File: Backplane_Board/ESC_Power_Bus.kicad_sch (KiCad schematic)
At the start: 19 parts, among them Q2 ZXMN3A14F, SW2 SW_DPST_x2

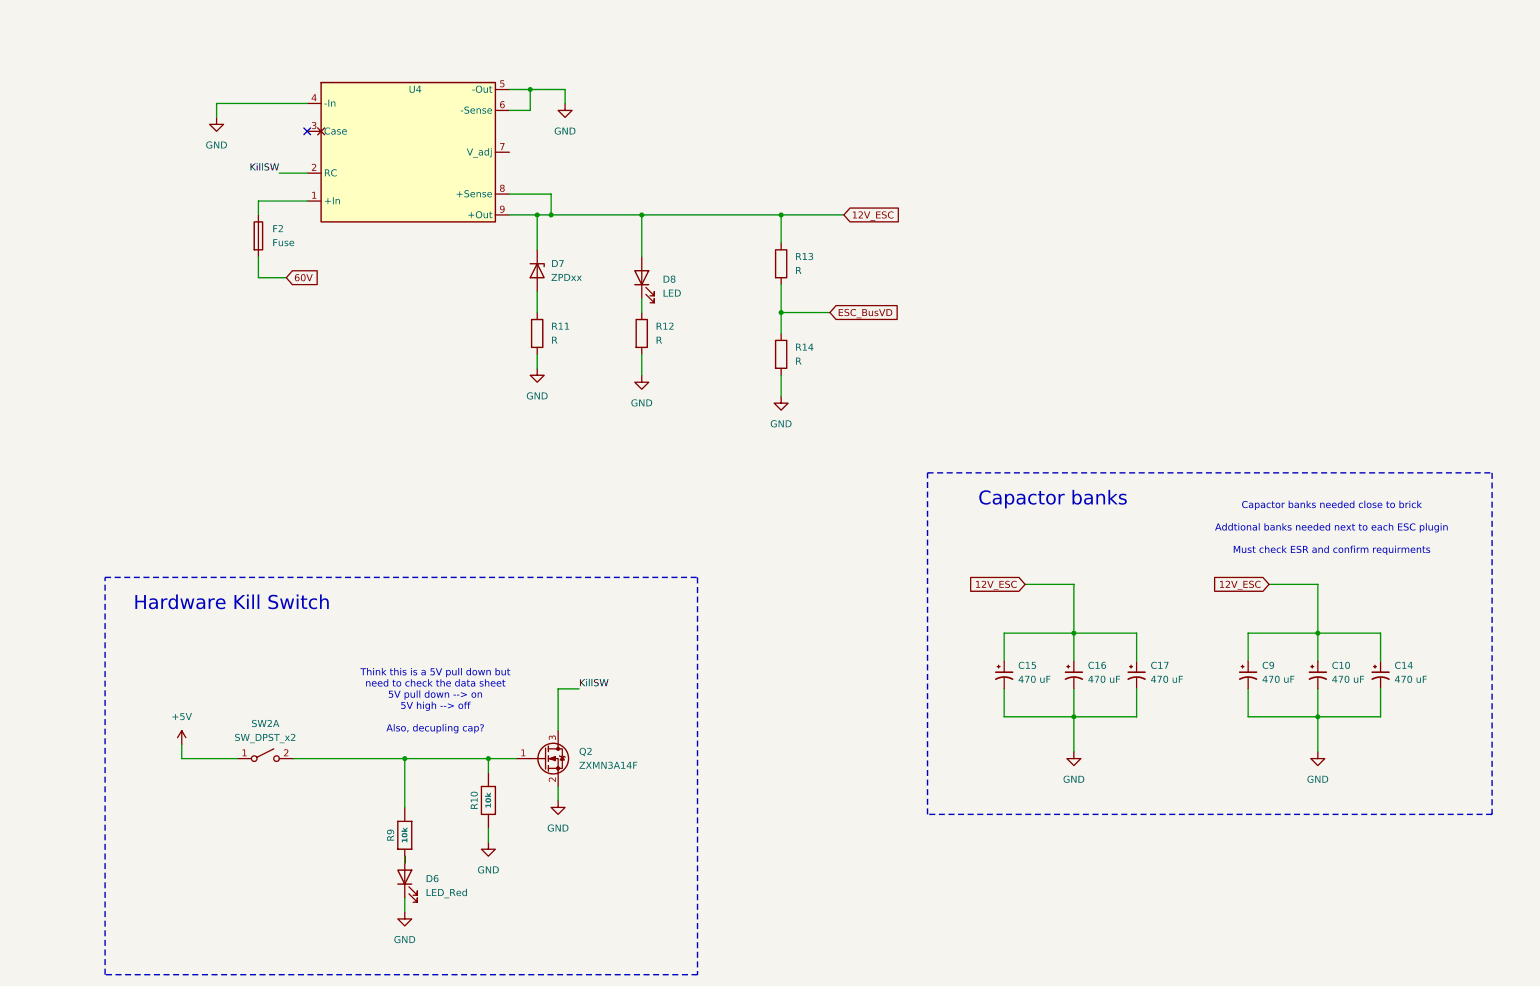
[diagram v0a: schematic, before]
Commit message: backup before heavy revtion
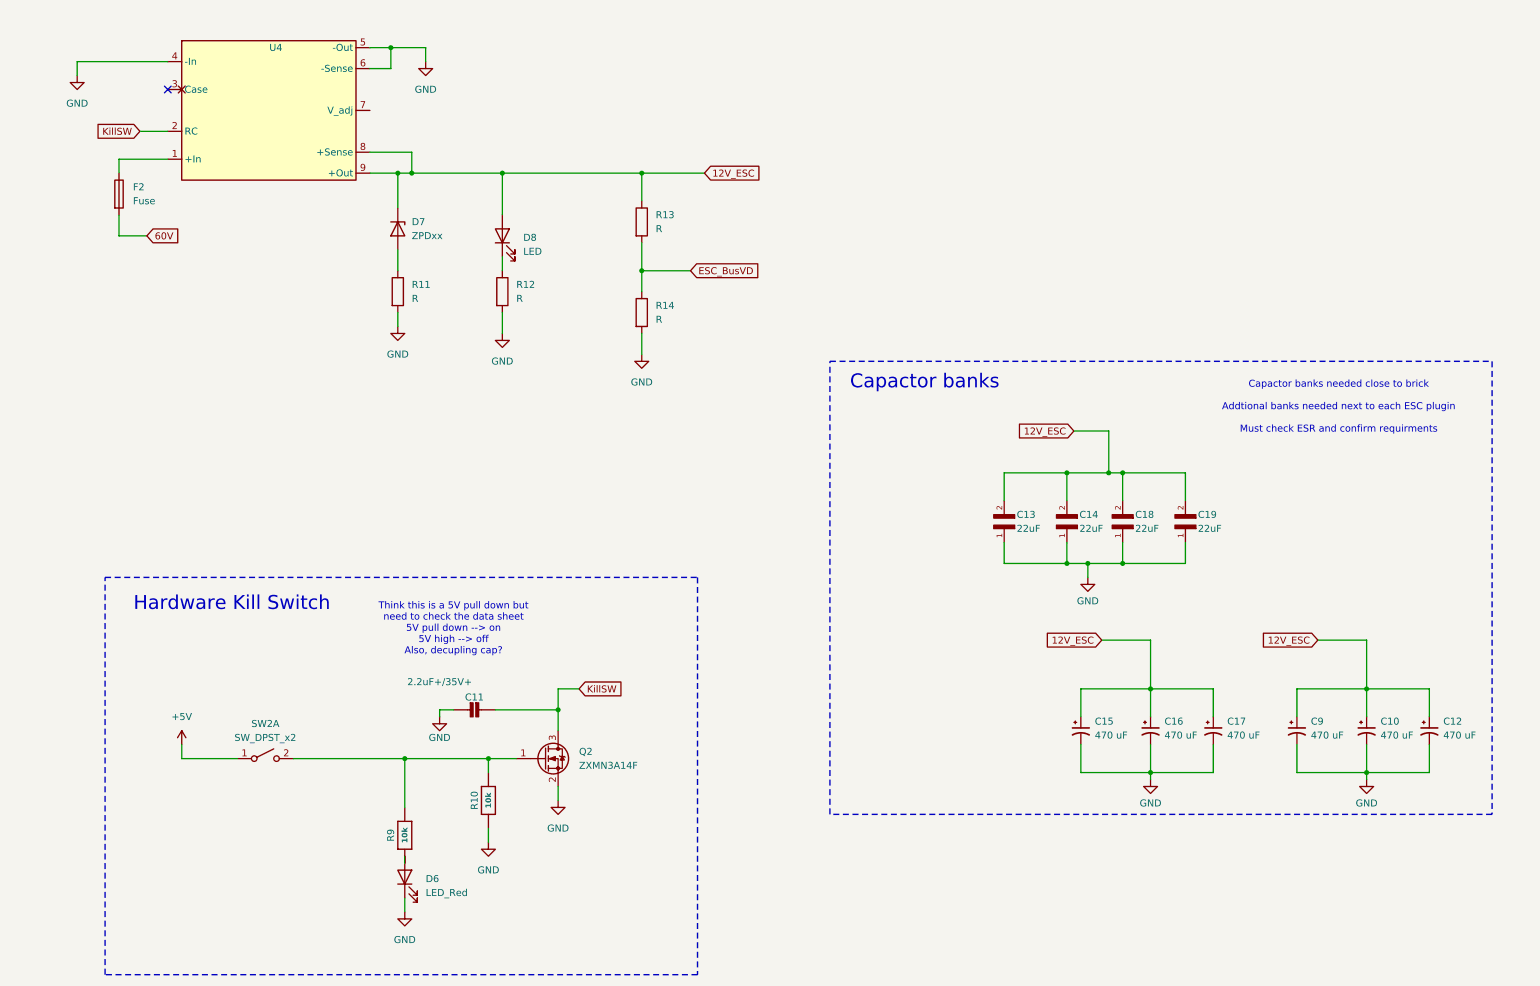
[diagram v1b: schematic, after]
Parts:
- removed C14: 470 uF, 470UF CAP:CAP_EEHZU1V471V, symbol Device:C_Polarized_Small_US
- added C11: 2.2uF+/35V+, Capacitor_SMD:C_0805_2012Metric, symbol Adafruit MOSFET Driver STEMMA Breakout-eagle-import:CAP_CERAMIC0805-NOOUTLINE
- added C12: 470 uF, 470UF CAP:CAP_EEHZU1V471V, symbol Device:C_Polarized_Small_US
- added C13, C14, C18, C19: 22uF, C2012X5R1V226M125AC:CAPC2012X145N, symbol C2012X5R1V226M125AC:C2012X5R1V226M125AC
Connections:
- net 12V_ESC: now also C12.1, C13.2, C14.2, C18.2, C19.2
- net GND: now also C11.2, C12.2, C13.1, C14.1, C18.1, C19.1
- net KillSW: now also C11.1
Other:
- moved on the sheet: C15, C16, C17, D7, D8, F2, R11, R12, R13, R14, U4

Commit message: back plane board ready for review
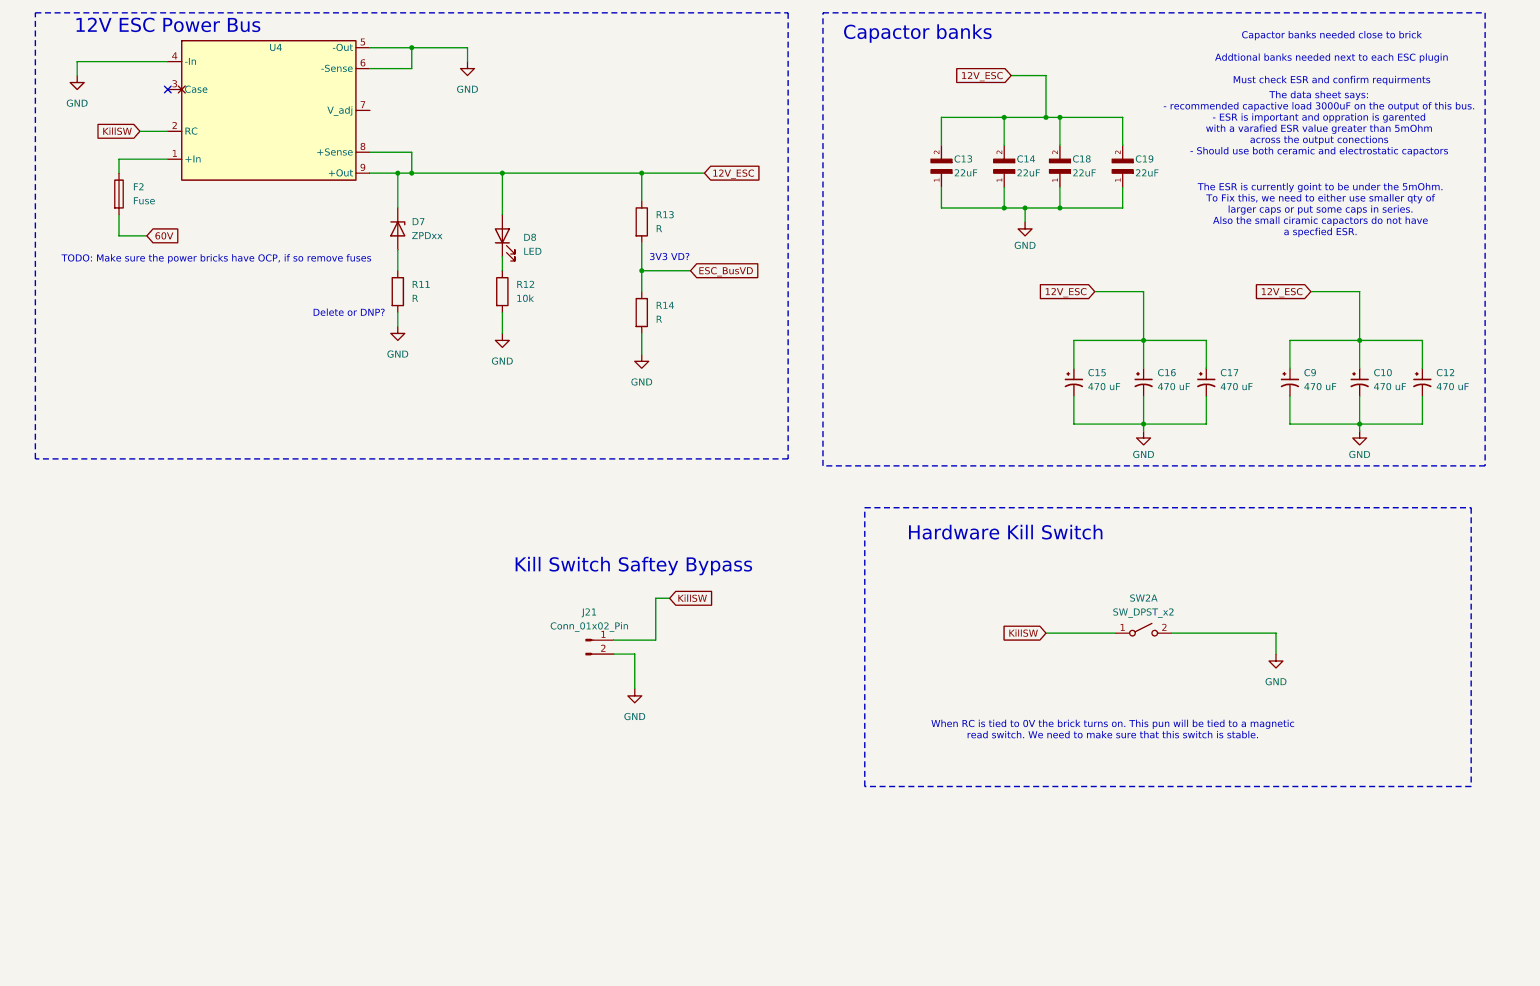
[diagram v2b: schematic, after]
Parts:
- removed C11: 2.2uF+/35V+, Capacitor_SMD:C_0805_2012Metric, symbol Adafruit MOSFET Driver STEMMA Breakout-eagle-import:CAP_CERAMIC0805-NOOUTLINE
- removed D6: LED_Red, LED_SMD:LED_0603_1608Metric, symbol Device:LED
- removed Q2: ZXMN3A14F, Package_TO_SOT_SMD:SOT-23, symbol Transistor_FET:ZXMN3A14F
- removed R10, R9: 10k, Resistor_SMD:R_0805_2012Metric, symbol Adafruit MOSFET Driver STEMMA Breakout-eagle-import:RESISTOR_0603_NOOUT
- added J21: Conn_01x02_Pin, symbol Connector:Conn_01x02_Pin
- R12: value R -> 10k
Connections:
- net +5V is gone; now on net KillSW: SW2.1 (A)
- net GND: now also SW2.2 (B), J21.2 (Pin_2)
- net KillSW: now also J21.1 (Pin_1)
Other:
- note added: "12V ESC Power Bus"
- note added: "3V3 VD?"
- note added: "Delete or DNP?"
- note added: "Kill Switch Saftey Bypass"
- note added: "TODO: Make sure the power bricks have OCP, if so remove fuses"
- note added: "The ESR is currently goint to be under the 5mOhm. To Fix this, we need to either use smaller qty of larger caps or put some caps in series. Also the small ciramic capactors do not have a specfied ESR."
- note added: "The data sheet says: - recommended capactive load 3000uF on the output of this bus. - ESR is important and oppration is garented with a varafied ESR value greater than 5mOhm across the output conections - Should use both ceramic and electrostatic capactors"
- note added: "When RC is tied to 0V the brick turns on. This pun will be tied to a magnetic read switch. We need to make sure that this switch is stable."
- note removed: "Think this is a 5V pull down but need to check the data sheet 5V pull down --> on 5V high --> off Also, decupling cap?"
- moved on the sheet: C10, C12, C13, C14, C15, C16, C17, C18, C19, C9, SW2A
